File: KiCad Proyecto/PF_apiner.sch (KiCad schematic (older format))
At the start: 7 parts, among them J1 OBDII Header, J2 Conn_01x05, U11 AZ1117EH-3.3TRG1

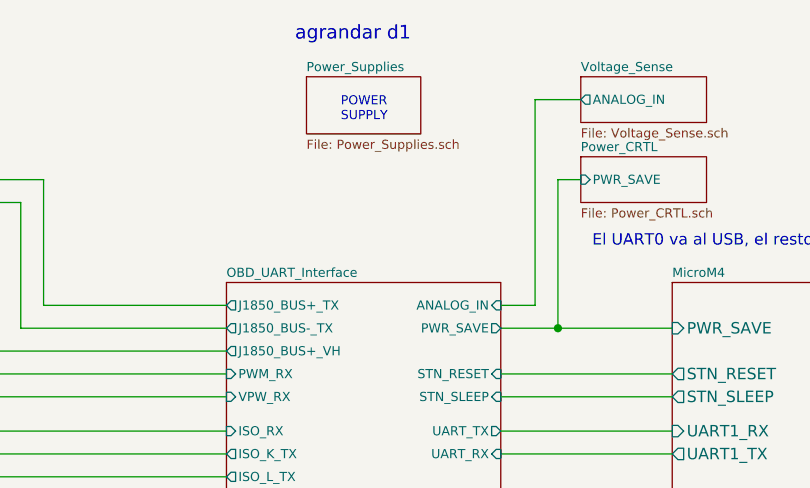
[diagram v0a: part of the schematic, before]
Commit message: ME curbas PF pos pcb
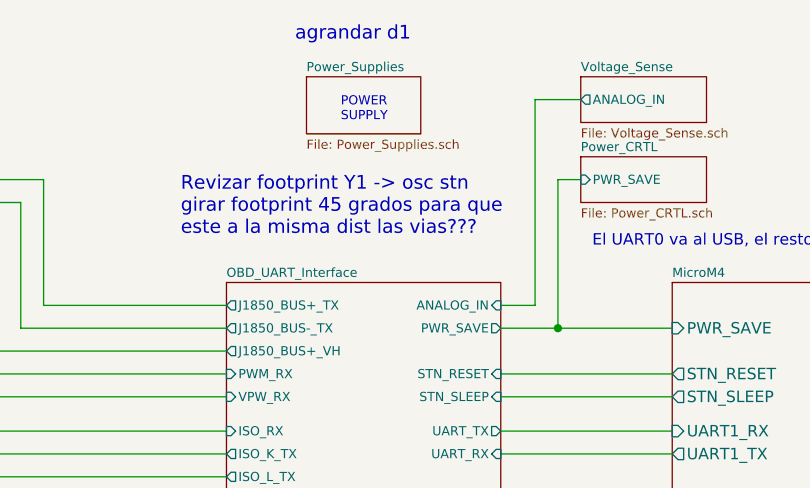
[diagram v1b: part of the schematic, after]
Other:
- note added: "Revizar footprint Y1 -> osc stn\ngirar footprint 45 grados para que \neste a la misma dist las vias???"
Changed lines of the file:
@@
 Text Notes 5400 1350 0    60   ~ 0
 agrandar d1
+Text Notes 4900 2200 0    60   ~ 0
+Revizar footprint Y1 -> osc stn\ngirar footprint 45 grados para que \neste a la misma dist las vias???
 $EndSCHEMATC

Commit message: modificado pcb
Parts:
- removed C34: 1uF, chip_rlc:c_0402, symbol C
- removed D11: MBR0520, to-sod-sot:SOD-123, symbol D_Schot
- removed U11: AZ1117EH-3.3TRG1, to-sod-sot:SOT-223, symbol VOLT_REG
- added H1, H2, H3, H4: PCB_HOLE, misc:MountingHole_3mm, symbol PCB_HOLE
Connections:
- net labels removed: +3.3V
- wire segments 114 -> 108
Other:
- note removed: "Revizar footprint Y1 -> osc stn\ngirar footprint 45 grados para que \neste a la misma dist las vias???"
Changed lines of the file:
@@
 LIBS:OBDII_IoT
 LIBS:STN2120
-LIBS:PF_apiner-cache
 EELAYER 25 0
 EELAYER END
@@
 $EndComp
 $Comp
-L VOLT_REG U?
-U 1 1 5B8838F5
-P 9550 4350
-AR Path="/582F2211/5B8838F5" Ref="U?"  Part="1"
-AR Path="/5B8838F5" Ref="U11"  Part="1"
-F 0 "U11" H 9400 4600 50  0000 C CNN
-F 1 "AZ1117EH-3.3TRG1" H 9575 4524 40  0000 C CNN
-F 2 "to-sod-sot:SOT-223" H 2000 -850 40  0001 C CNN
-F 3 "" H 2000 -850 40  0000 C CNN
-F 4 "IC REG LDO 3.3V 1A SOT223" H 9550 4350 60  0001 C CNN "Desc"
-F 5 "Diodes Incorporated" H 9550 4350 60  0001 C CNN "Manf"
-F 6 "AZ1117EH-3.3TRG1" H 9550 4350 60  0001 C CNN "Manf#"
-F 7 "AZ1117EH-3.3TRG1DICT-ND" H 9550 4350 60  0001 C CNN "Digikey#"
-	1    9550 4350
-	-1   0    0    -1
-$EndComp
-$Comp
-L C C?
-U 1 1 5B883906
-P 9050 4600
-AR Path="/582F2211/5B883906" Ref="C?"  Part="1"
-AR Path="/5B883906" Ref="C34"  Part="1"
-F 0 "C34" V 8950 4550 50  0000 L CNN
-F 1 "1uF" V 9150 4500 50  0000 L CNN
-F 2 "chip_rlc:c_0402" H 9088 4450 50  0001 C CNN
-F 3 "" H 9050 4600 50  0000 C CNN
-F 4 "CAP CER 1UF 6.3V X5R 0402" H 9050 4600 60  0001 C CNN "Desc"
-F 5 "Taiyo Yuden" H 9050 4600 60  0001 C CNN "Manf"
-F 6 "JMK105BJ105KV-F" H 9050 4600 60  0001 C CNN "Manf#"
-F 7 "587-1231-1-ND" H 9050 4600 60  0001 C CNN "Digikey#"
-	1    9050 4600
-	-1   0    0    -1
-$EndComp
-$Comp
-L +3.3V #PWR?
-U 1 1 5B88390D
-P 8500 4250
-AR Path="/582F2211/5B88390D" Ref="#PWR?"  Part="1"
-AR Path="/5B88390D" Ref="#PWR03"  Part="1"
-F 0 "#PWR03" H 8550 4300 20  0001 C CNN
-F 1 "+3.3V" H 8500 4350 30  0000 C CNN
-F 2 "" H 1750 -450 60  0000 C CNN
-F 3 "" H 1750 -450 60  0000 C CNN
-	1    8500 4250
-	-1   0    0    -1
-$EndComp
-$Comp
-L GND #PWR?
-U 1 1 5B883913
-P 9550 4850
-AR Path="/582F2211/5B883913" Ref="#PWR?"  Part="1"
-AR Path="/5B883913" Ref="#PWR04"  Part="1"
-F 0 "#PWR04" H 9550 4600 50  0001 C CNN
-F 1 "GND" H 9550 4700 50  0001 C CNN
-F 2 "" H 9550 4850 50  0000 C CNN
-F 3 "" H 9550 4850 50  0000 C CNN
-	1    9550 4850
-	-1   0    0    -1
-$EndComp
-$Comp
 L GND #PWR?
 U 1 1 5B883919
 P 10000 4850
 AR Path="/582F2211/5B883919" Ref="#PWR?"  Part="1"
-AR Path="/5B883919" Ref="#PWR05"  Part="1"
-F 0 "#PWR05" H 10000 4600 50  0001 C CNN
+AR Path="/5B883919" Ref="#PWR03"  Part="1"
+F 0 "#PWR03" H 10000 4600 50  0001 C CNN
 F 1 "GND" H 10000 4700 50  0001 C CNN
 F 2 "" H 10000 4850 50  0000 C CNN
@@
 $EndComp
 $Comp
-L GND #PWR?
-U 1 1 5B88391F
-P 9050 4850
-AR Path="/582F2211/5B88391F" Ref="#PWR?"  Part="1"
-AR Path="/5B88391F" Ref="#PWR06"  Part="1"
-F 0 "#PWR06" H 9050 4600 50  0001 C CNN
-F 1 "GND" H 9050 4700 50  0001 C CNN
-F 2 "" H 9050 4850 50  0000 C CNN
-F 3 "" H 9050 4850 50  0000 C CNN
-	1    9050 4850
-	-1   0    0    -1
-$EndComp
-$Comp
-L +5V_USB #U07
+L +5V_USB #U04
 U 1 1 5B88F65F
 P 9250 2300
-F 0 "#U07" H 9250 2450 50  0001 C CNN
+F 0 "#U04" H 9250 2450 50  0001 C CNN
 F 1 "+5V_USB" H 9050 2450 30  0000 L CNN
 F 2 "" H 9250 2300 50  0001 C CNN
@@
 P 10000 4250
 AR Path="/5B89C1C4/5B8A5F5E" Ref="#PWR?"  Part="1"
-AR Path="/5B8A5F5E" Ref="#PWR08"  Part="1"
-F 0 "#PWR08" H 10000 4340 20  0001 C CNN
+AR Path="/5B8A5F5E" Ref="#PWR05"  Part="1"
+F 0 "#PWR05" H 10000 4340 20  0001 C CNN
 F 1 "+5V" H 10000 4340 30  0000 C CNN
 F 2 "" H 10000 4250 60  0000 C CNN
@@
 P 10650 4250
 AR Path="/5B89C1C4/5B8A5F68" Ref="U?"  Part="1"
-AR Path="/5B8A5F68" Ref="#U09"  Part="1"
-F 0 "#U09" H 10650 4400 50  0001 C CNN
+AR Path="/5B8A5F68" Ref="#U06"  Part="1"
+F 0 "#U06" H 10650 4400 50  0001 C CNN
 F 1 "+5V_USB" H 10697 4279 30  0000 L CNN
 F 2 "" H 10650 4250 50  0001 C CNN
@@
 $EndComp
 $Comp
-L D_Schot D?
-U 1 1 5B8B67B7
-P 8850 4350
-AR Path="/5B89C1C4/5B8B67B7" Ref="D?"  Part="1"
-AR Path="/5B8B67B7" Ref="D11"  Part="1"
-F 0 "D11" H 8800 4430 50  0000 L CNN
-F 1 "MBR0520" H 8730 4250 40  0000 L CNN
-F 2 "to-sod-sot:SOD-123" V 8850 4350 50  0001 C CNN
-F 3 "" V 8850 4350 50  0000 C CNN
-F 4 "DIODE SCHOTTKY 20V 500MA SOD123" H 8850 4350 50  0001 C CNN "Desc"
-F 5 "ON Semiconductor" H 8850 4350 50  0001 C CNN "Manf"
-F 6 "MBR0520LT1G" H 8850 4350 50  0001 C CNN "Manf#"
-F 7 "MBR0520LT1GOSCT-ND" H 8850 4350 50  0001 C CNN "Digikey#"
-	1    8850 4350
-	1    0    0    -1
-$EndComp
-$Comp
 L GND #PWR?
 U 1 1 5B8BA0D1
 P 8900 3050
 AR Path="/582F2211/5B8BA0D1" Ref="#PWR?"  Part="1"
-AR Path="/5B8BA0D1" Ref="#PWR010"  Part="1"
-F 0 "#PWR010" H 8900 2800 50  0001 C CNN
+AR Path="/5B8BA0D1" Ref="#PWR07"  Part="1"
+F 0 "#PWR07" H 8900 2800 50  0001 C CNN
 F 1 "GND" H 8900 2900 50  0001 C CNN
 F 2 "" H 8900 3050 50  0000 C CNN
@@
 $EndComp
 $Comp
-L PWR_FLAG #FLG011
+L PWR_FLAG #FLG08
 U 1 1 5BA598FF
 P 9350 2200
-F 0 "#FLG011" H 9350 2295 50  0001 C CNN
+F 0 "#FLG08" H 9350 2295 50  0001 C CNN
 F 1 "PWR_FLAG" H 9350 2380 40  0000 C CNN
 F 2 "" H 9350 2200 50  0000 C CNN
@@
 	10000 4250 10000 4450
 Wire Wire Line
-	9950 4350 10250 4350
-Wire Wire Line
 	10000 4750 10000 4850
-Wire Wire Line
-	9550 4800 9550 4850
-Wire Wire Line
-	9050 4850 9050 4750
-Wire Wire Line
-	8950 4350 9100 4350
 Wire Wire Line
 	9250 2300 9250 2400
@@
 Connection ~ 10000 4350
 Wire Wire Line
-	8500 4250 8500 4350
-Wire Wire Line
-	8500 4350 8750 4350
-Wire Wire Line
 	8900 2900 9350 2900
 Wire Wire Line
@@
 Wire Wire Line
 	9350 2200 9350 2500
-Wire Wire Line
-	9050 4450 9050 4350
-Connection ~ 9050 4350
 $Comp
 L Conn_01x05 J2
@@
 Text Notes 5400 1350 0    60   ~ 0
 agrandar d1
-Text Notes 4900 2200 0    60   ~ 0
-Revizar footprint Y1 -> osc stn\ngirar footprint 45 grados para que \neste a la misma dist las vias???
+Wire Wire Line
+	10000 4350 10250 4350
+$Comp
+L PCB_HOLE H4
+U 1 1 5BDBC2D4
+P 10050 3650
+F 0 "H4" H 9900 3650 60  0000 C CNN
+F 1 "PCB_HOLE" H 10350 3650 60  0000 C CNN
+F 2 "misc:MountingHole_3mm" H 9900 3700 60  0001 C CNN
+F 3 "PCB HOLE" H 10000 3800 60  0001 C CNN
+	1    10050 3650
+	1    0    0    -1
+$EndComp
+$Comp
+L PCB_HOLE H3
+U 1 1 5BDBD6A0
+P 10050 3500
+F 0 "H3" H 9900 3500 60  0000 C CNN
+F 1 "PCB_HOLE" H 10350 3500 60  0000 C CNN
+F 2 "misc:MountingHole_3mm" H 9900 3550 60  0001 C CNN
+F 3 "PCB HOLE" H 10000 3650 60  0001 C CNN
+	1    10050 3500
+	1    0    0    -1
+$EndComp
+$Comp
+L PCB_HOLE H2
+U 1 1 5BDBD82A
+P 10050 3350
+F 0 "H2" H 9900 3350 60  0000 C CNN
+F 1 "PCB_HOLE" H 10350 3350 60  0000 C CNN
+F 2 "misc:MountingHole_3mm" H 9900 3400 60  0001 C CNN
+F 3 "PCB HOLE" H 10000 3500 60  0001 C CNN
+	1    10050 3350
+	1    0    0    -1
+$EndComp
+$Comp
+L PCB_HOLE H1
+U 1 1 5BDBD9BA
+P 10050 3200
+F 0 "H1" H 9900 3200 60  0000 C CNN
+F 1 "PCB_HOLE" H 10350 3200 60  0000 C CNN
+F 2 "misc:MountingHole_3mm" H 9900 3250 60  0001 C CNN
+F 3 "PCB HOLE" H 10000 3350 60  0001 C CNN
+	1    10050 3200
+	1    0    0    -1
+$EndComp
 $EndSCHEMATC
